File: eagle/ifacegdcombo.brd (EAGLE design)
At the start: 231.4 x 133.3 mm, 60 parts, among them IC1 ISO1540, K1 G5V-2, T1 TIP122V, T3 TIP122V, X1 BU-SMA-V, X4 BU-SMA-V

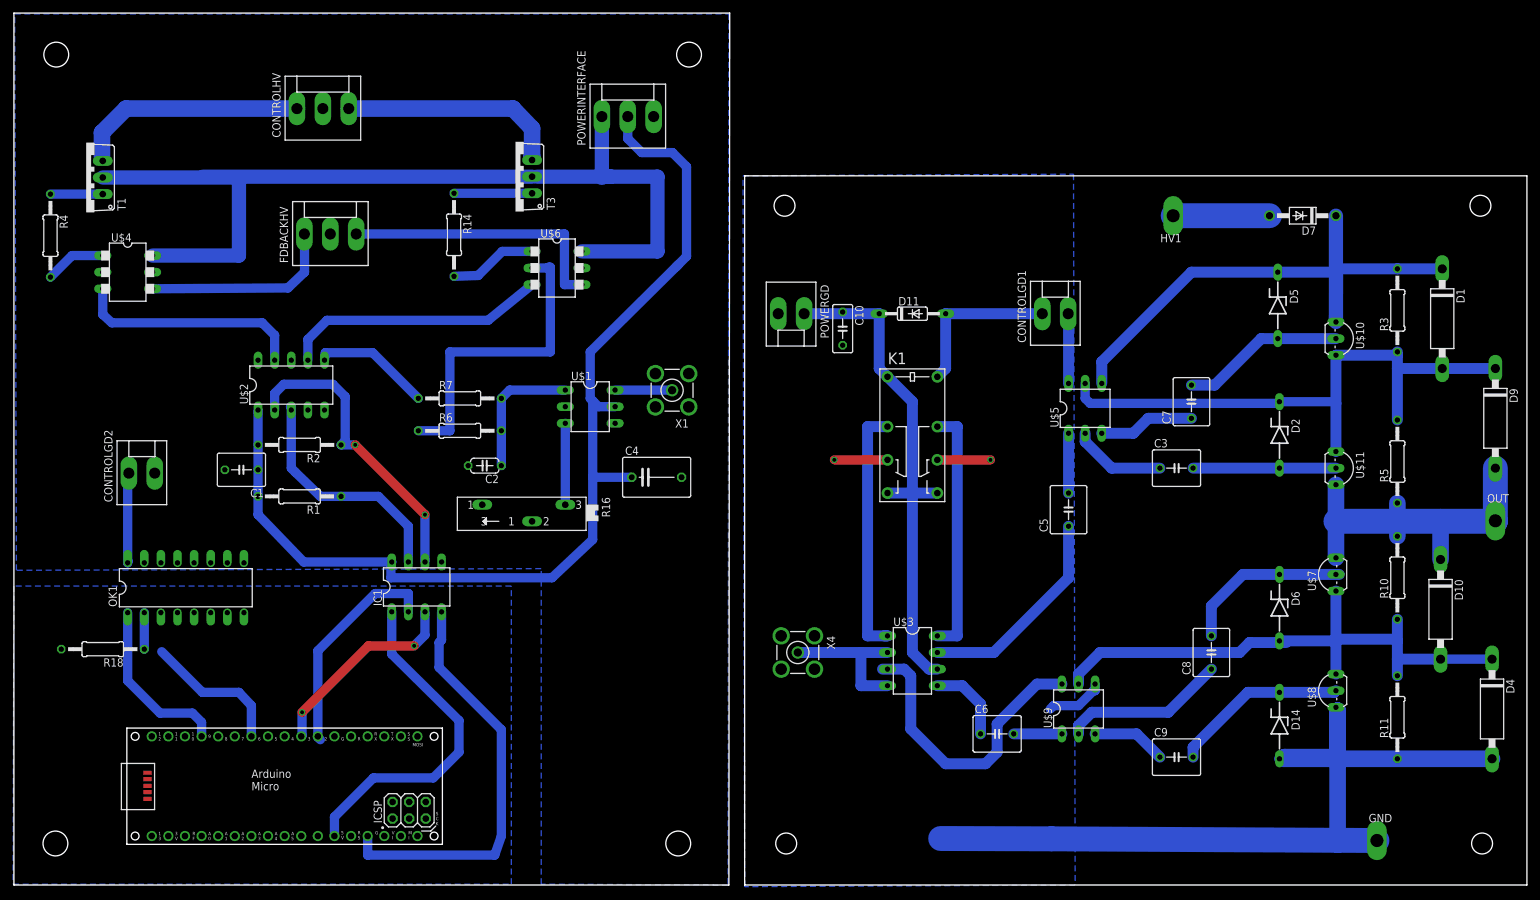
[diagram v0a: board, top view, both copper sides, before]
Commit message: IXYS board solution, gatedriver components
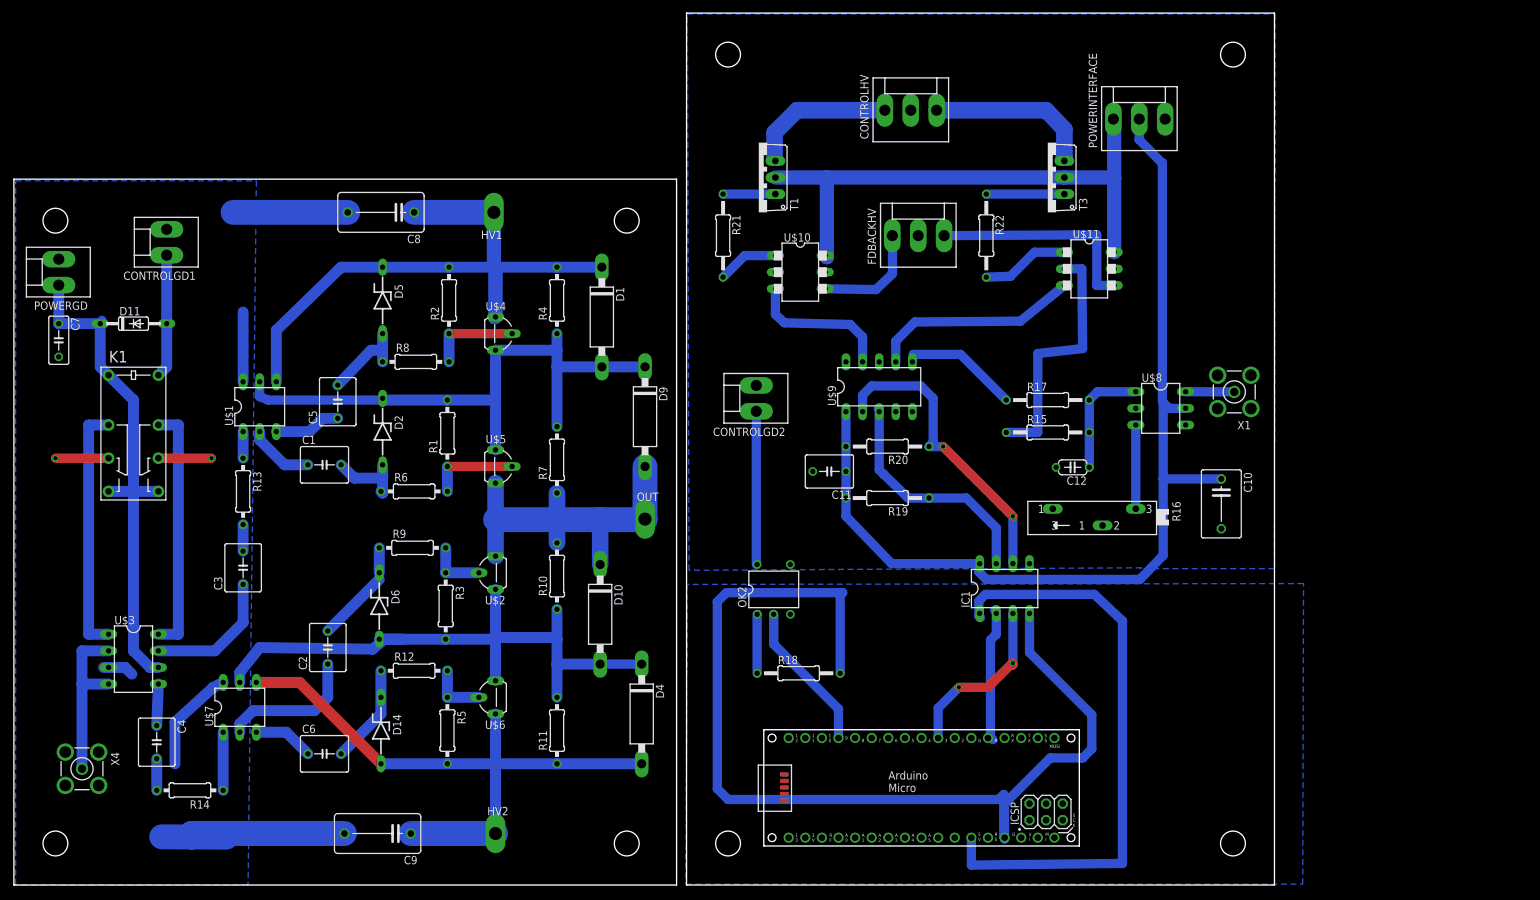
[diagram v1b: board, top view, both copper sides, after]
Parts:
- removed D7: 1N4004, diode:DO41-10
- removed GND: TPPAD1-20Y, testpad:P1-20Y
- removed OK1: PS2501", optocoupler:DIL16
- added C11: (no value), rcl:C050-050X075
- added C12: 10n, resistor:C050-024X044
- added HV2: TPPAD1-20Y, testpad:P1-20Y
- added OK2: H11F1, optocoupler:DIL05
- added R12, R13, R8, R9: 70, rcl:0207/10
- added R15: 10k, resistor:0207/12
- added R17: 40k, resistor:0207/12
- added R19, R20: 1.5k, resistor:0207/12
- added R21, R22: 1k, resistor:0207/12
- C1: value (none) -> .22u; device rcl:C050-050X075 -> resistor:C050-055X075
- C10: device rcl:C050-030X075 -> resistor:C075-063X106
- C2: value 10n -> .22u; device resistor:C050-024X044 -> resistor:C050-055X075
- C3, C5, C6: value (none) -> .22u
- C4: value (none) -> .22u; device resistor:C075-063X106 -> resistor:C050-055X075
- C7: device resistor:C050-055X075 -> rcl:C050-030X075
- C8, C9: value (none) -> 10p; device resistor:C050-055X075 -> resistor:C102-064X133
- R1, R2: value 1.5k -> 50k; device resistor:0207/12 -> rcl:0207/10
- R10, R11: value 10M -> 1M; device rcl:0207/12 -> rcl:0207/10
- R14, R4: value 1k -> 1M; device resistor:0207/12 -> rcl:0207/10
- R3, R5: value 10M -> 50k; device rcl:0207/12 -> rcl:0207/10
- R6: value 10k -> 70; device resistor:0207/12 -> rcl:0207/10
- R7: value 40k -> 1M; device resistor:0207/12 -> rcl:0207/10
- U$1: value LTC6992 -> DA-2320; device linear-technology:DIL06 -> trafo:DIL06
- U$10, U$11: value VP0550 -> MAX9650DIL; device transistor-fet:TO92- -> maxim:DIL06-4
- U$2: value MCP4728DIL -> VN0550L; device microchip:DIL10 -> transistor-fet:TO92L
- U$4: value MAX9650DIL -> VP0550L; device maxim:DIL06-4 -> transistor-fet:TO92L
- U$5: value DA-2320 -> VP0550L; device trafo:DIL06 -> transistor-fet:TO92L
- U$6: value MAX9650DIL -> VN0550L; device maxim:DIL06-4 -> transistor-fet:TO92L
- U$7: value VN0550 -> DA-2320; device transistor-fet:TO92- -> trafo:DIL06
- U$8: value VN0550 -> LTC6992; device transistor-fet:TO92- -> linear-technology:DIL06
- U$9: value DA-2320 -> MCP4728DIL; device trafo:DIL06 -> microchip:DIL10
- moved C7 173.5 mm to (6.86, 83.3), turned to 270 degrees
- moved U$7 168.9 mm to (34.5, 27.2), turned to 0 degrees
- moved R3 152.4 mm to (66.0, 42.7), turned to 270 degrees
- moved R5 151.0 mm to (66.3, 23.6), turned to 270 degrees
- moved C8 143.7 mm to (56.1, 102.9), turned to 180 degrees
- moved C3 143.6 mm to (35.1, 48.5), turned to 90 degrees
- moved D6 137.7 mm to (55.9, 42.7)
- moved D14 137.4 mm to (56.1, 23.6)
- moved D2 137.2 mm to (56.4, 69.3)
- moved D5 136.9 mm to (56.4, 89.4)
- moved CONTROLGD1 136.3 mm to (23.4, 98.3), turned to 90 degrees
- moved D4 130.1 mm to (96.0, 26.2)
- moved D9 130.0 mm to (96.5, 71.6)
- moved OUT 130.0 mm to (96.5, 56.0)
- moved R11 128.5 mm to (83.1, 23.6)
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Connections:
- removed net N$1 (its old number): R7.1, U$2.6
- removed net N$14 (its old number): FDBACKHV.3, U$6.4
- removed net N$15 (its old number): R14.1, T3.1
- new net N$20: C4.2, R14.2
- new net N$22: C2.1, U$7.2
- new net N$23: C6.1, U$7.3
- new net N$251: R3.1, R9.2, U$2.2
- new net N$39: R22.2, U$11.1
- new net N$4: C4.1, U$3.5
- new net N$43: R21.1, T1.1
- new net N$5: C1.1, U$1.2
- new net N$6: R14.1, U$7.1
- net +12V: now also U$10.6, U$11.6; no longer U$4.6, U$6.6
- net +15V: now also C7.1; no longer C10.1
- net ENSW2: now also OK2.6; no longer OK1.16
- net GND: now also C7.2, C8.2, C9.2, CONTROLGD1.2, K1.11, K1.6, POWERGD.2, U$1.6, U$3.3, U$7.6, X4.2, X4.3, X4.4, X4.5; no longer C1.2, C2.2, C4.2, CONTROLGD2.2, CONTROLHV.2, FDBACKHV.2, IC1.5, OK1.15, POWERINTERFACE.3, R16.A, R16.S, R6.1, U$1.DIV, U$1.GND, U$2.10, U$2.4, U$4.2, U$6.2, X1.2, X1.3, X1.4, X1.5
- net GND1: now also C11.2, C12.2, CONTROLGD2.2, CONTROLHV.2, FDBACKHV.2, IC1.5, OK2.4, POWERINTERFACE.3, R15.1, R16.A, R16.S, U$10.2, U$11.2, U$8.DIV, U$8.GND, U$9.10, X1.2, X1.3, X1.4, X1.5; no longer CONTROLGD1.2, D14.A, D4.A, GND.TP, K1.11, K1.6, POWERGD.2, R11.1, U$3.3, U$5.6, U$8.3, U$9.6, X4.2, X4.3, X4.4, X4.5
- net N$10: now also C1.2, D2.A, R6.1; no longer C5.1, U$3.7
- net N$11: now also R12.2, R5.1, U$6.2; no longer C6.1, U$3.5
- net N$12: now also R2.1, R8.2, U$4.2; no longer R16.E, U$1.SET
- net N$13: now also D10.A, D4.C, D6.A, R10.1, R11.2, R3.2, U$2.3, U$6.1; no longer U$1.OUT, X1.1
- net N$16: now also C5.2, D5.A, R8.1; no longer U$2.9, U$4.3
- net N$17: now also C8.1, D1.C, D5.C, HV1.TP, R2.2, R4.2, U$1.4, U$4.3; no longer U$2.8
- net N$18: now also D1.A, D2.C, D9.C, R1.2, R4.1, R7.2, U$1.5, U$4.1, U$5.3; no longer U$2.7, U$6.3
- net N$19: now also C3.2, R13.2; no longer R4.2, U$4.1
- net N$2: now also C3.1, U$3.7; no longer C2.1, R6.2, R7.2, U$1.MOD
- net N$21: now also D10.C, D9.A, OUT.TP, R10.2, R7.1, U$2.1, U$5.1; no longer R14.2, U$6.1
- net N$24: now also C9.1, D14.A, D4.A, HV2.TP, R11.1, R5.2, U$6.3, U$7.4; no longer C3.1, U$5.2
- net N$25: now also C2.2, D6.C, R9.1; no longer C7.1, U$5.3
- net N$26: now also R16.E, U$8.SET; no longer C8.1, U$9.2
- net N$27: now also C6.2, D14.C, R12.1; no longer C9.1, U$9.3
- net N$28: now also U$8.OUT, X1.1; no longer C8.2, D6.C, U$7.2
- net N$29: now also OK2.1, R18.1; no longer C9.2, D14.C, U$8.2
- net N$3: now also R13.1, U$1.1; no longer R4.1, T1.1
- net N$30: now also C12.1, R15.2, R17.2, U$8.MOD; no longer C3.2, D2.A, U$11.2
- net N$31: now also FDBACKHV.1, U$10.4; no longer C7.2, D5.A, U$10.2
- net N$32: now also FDBACKHV.3, U$11.4; no longer D1.C, D5.C, D7.C, R3.2, U$10.3, U$5.4
- net N$33: now also U$10.3, U$9.9; no longer D10.C, D9.A, OUT.TP, R10.2, R5.1, U$11.1, U$7.1
- net N$34: now also U$9.8; no longer D7.A, HV1.TP
- net N$35: now also U$11.3, U$9.7; no longer C6.2, U$9.1
- net N$36: now also R17.1, U$9.6; no longer U$9.5
- net N$37: now also R22.1, T3.1; no longer D10.A, D4.C, D6.A, R10.1, R11.2, U$7.3, U$8.1
- net N$38: now also R21.2; no longer D1.A, D2.C, D9.C, R3.1, R5.2, U$11.3, U$5.5
- net N$7: now also C5.1, U$1.3; no longer OK1.2, R18.1
- net N$8: now also R1.1, R6.2, U$5.2; no longer FDBACKHV.1, U$4.4
- net N$9: now also U$7.5; no longer C5.2, U$5.1
- net PWM9: now also OK2.2; no longer OK1.1
- net SCL_OUT: now also R20.1, U$9.2; no longer R2.1, U$2.2
- net SDA_OUT: now also R19.1, U$9.3; no longer R1.1, U$2.3
- net VCC: now also C10.1, C11.1, R19.2, R20.2, U$8.VCC, U$9.1; no longer C1.1, C4.1, R1.2, R2.2, U$1.VCC, U$2.1
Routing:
- net GND1: track 215.9 -> 38.7 mm, vias 2 -> 0
- net N$17: track 0.00 -> 98.4 mm
- net AGND: track 63.8 -> 159.2 mm
- net N$38: track 90.7 -> 9.37 mm
- net N$24: track 14.4 -> 95.6 mm
- net +12V: track 149.3 -> 84.8 mm
- net N$18: track 40.6 -> 100.8 mm
- net N$13: track 8.72 -> 68.3 mm
- net N$32: track 85.7 -> 33.8 mm
- net GND: track 48.1 -> 98.9 mm, vias 0 -> 2
- net N$37: track 55.6 -> 11.9 mm
- net N$21: track 13.5 -> 56.6 mm
- net N$14 (its old number): track 42.3 -> 0.00 mm
- net A+5: track 51.8 -> 91.0 mm
- net N$33: track 54.6 -> 22.4 mm
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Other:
- board size 231.4 x 133.3 mm -> 192.8 x 133.3 mm
